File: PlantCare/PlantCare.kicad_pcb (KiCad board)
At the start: 2 copper layers, 27 parts, among them J1 USB4105-GF-A, SW1 PTS810_SJM_250_SMTR_LFS, SW2 PTS810_SJM_250_SMTR_LFS, U1 AMS1117-3.3, U2 ESP32-S3-WROOM-1-N16R2

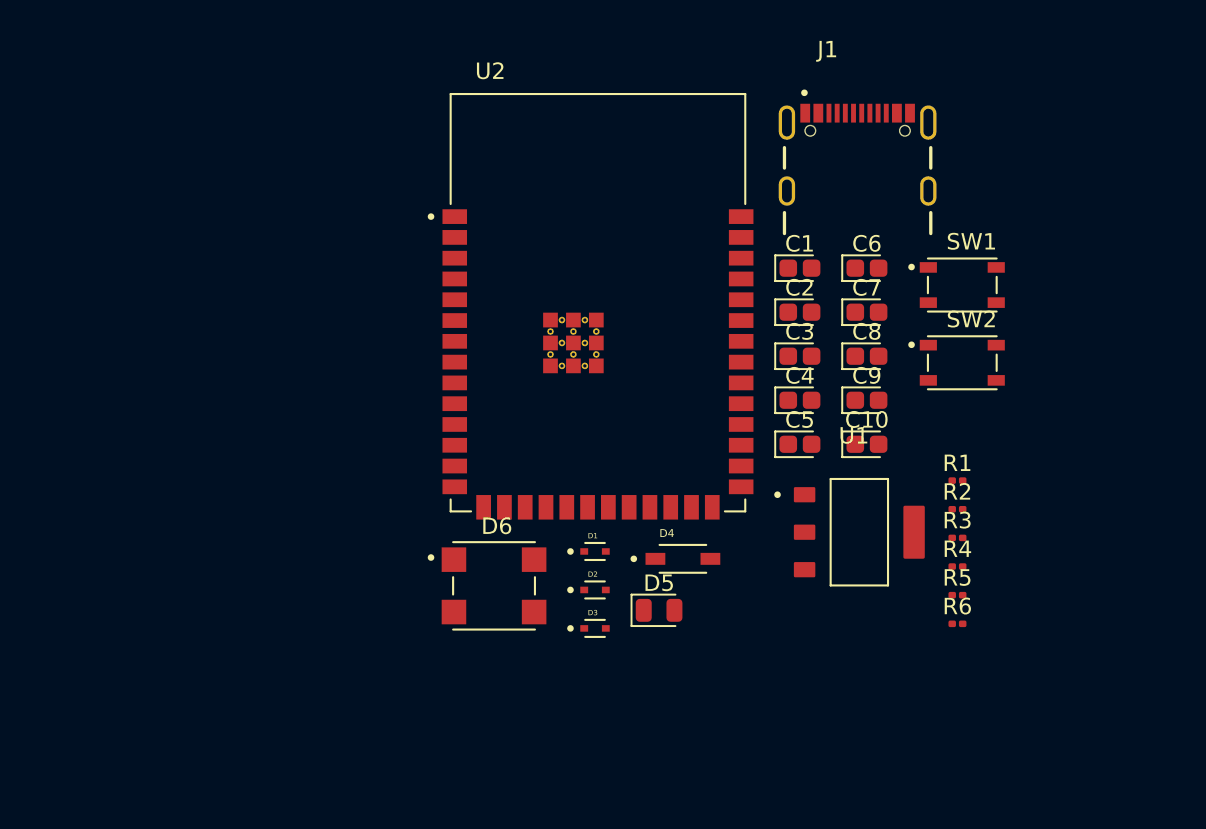
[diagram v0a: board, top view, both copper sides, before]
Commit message: Clear pcb
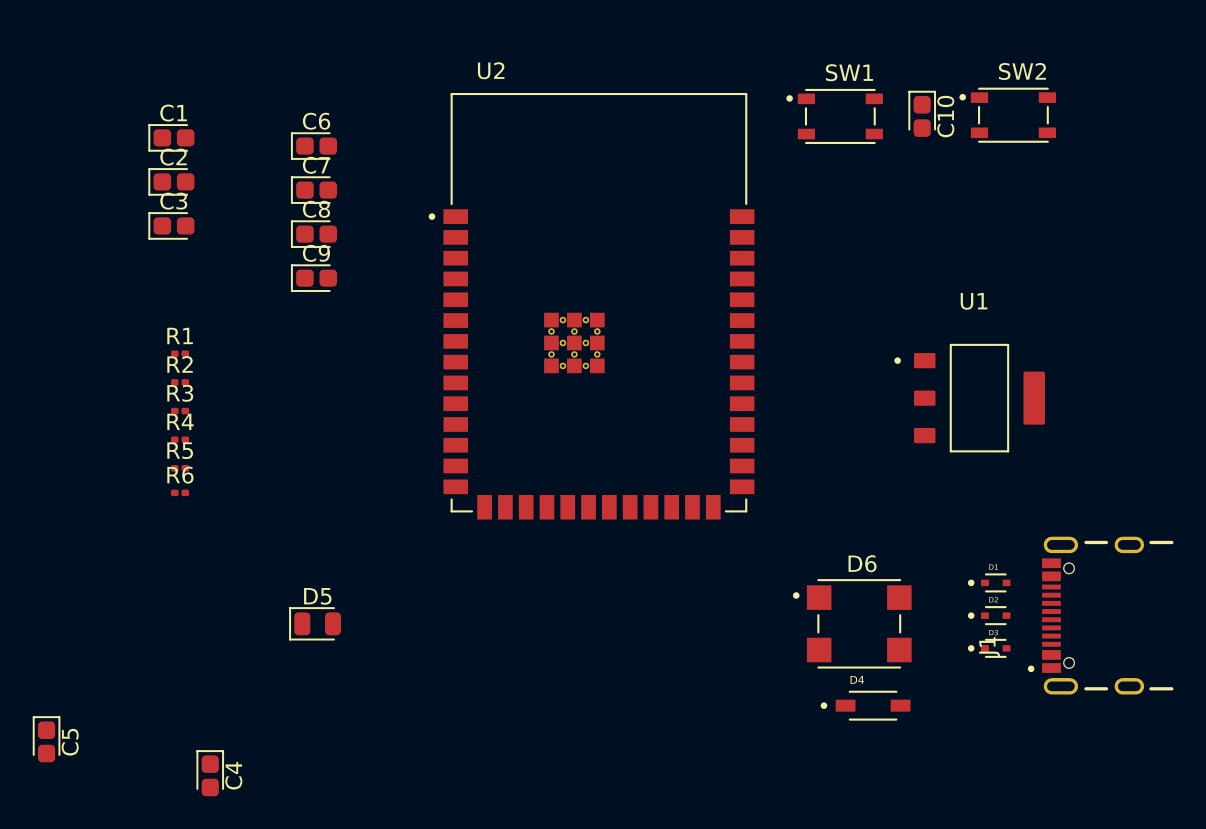
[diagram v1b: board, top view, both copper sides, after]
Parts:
- moved C5 49.5 mm to (111.5, 112.2), turned to -90 degrees
- moved R6 48.2 mm to (119.7, 97.0)
- moved R1 48.1 mm to (119.7, 88.5)
- moved R2 48.1 mm to (119.7, 90.2)
- moved R3 48.1 mm to (119.7, 92.0)
- moved R4 48.1 mm to (119.7, 93.8)
- moved R5 48.1 mm to (119.7, 95.5)
- moved C4 42.7 mm to (121.5, 114.3), turned to -90 degrees
- moved C3 39.1 mm to (119.3, 80.7)
- moved C1 39.1 mm to (119.3, 75.3)
- moved C2 39.1 mm to (119.3, 78.0)
- moved C8 34.4 mm to (128.0, 81.2)
- moved C9 34.4 mm to (128.0, 83.9)
- moved C6 34.4 mm to (128.0, 75.8)
- moved C7 34.4 mm to (128.0, 78.5)
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
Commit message: Fix pc
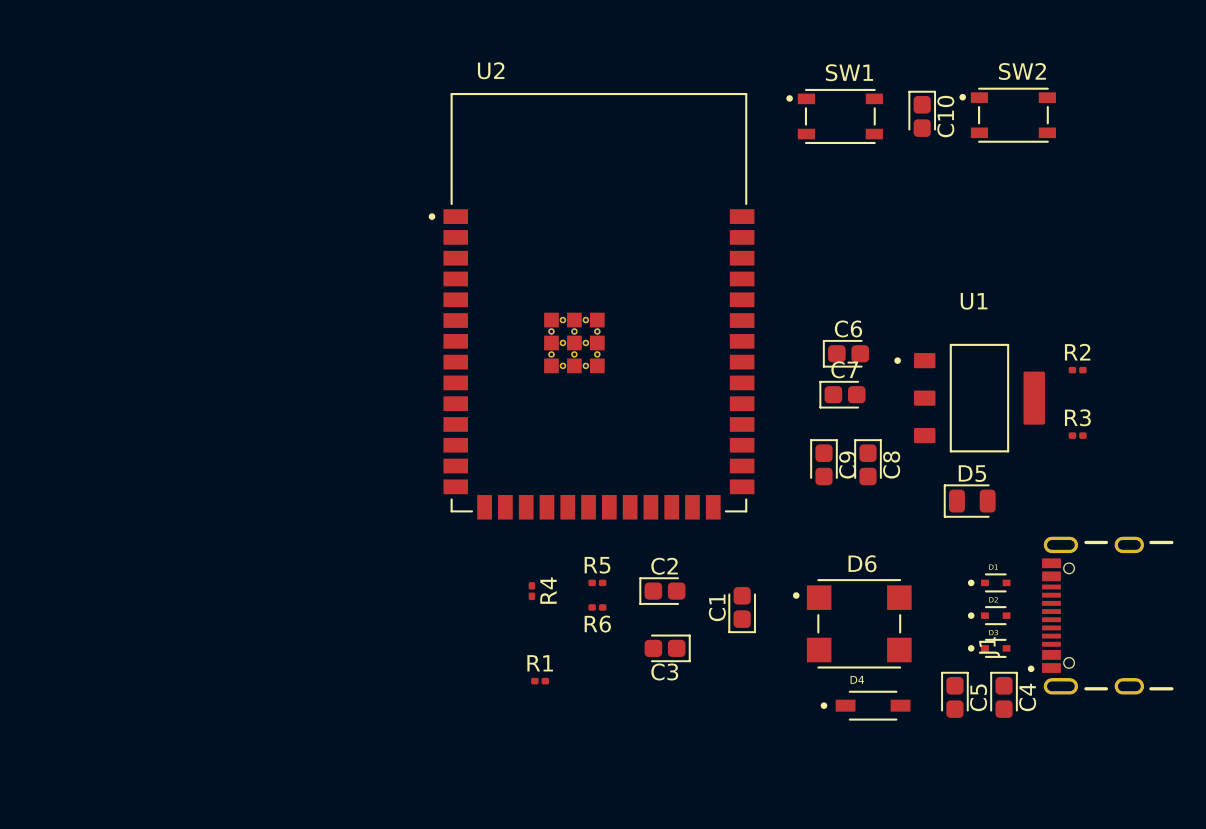
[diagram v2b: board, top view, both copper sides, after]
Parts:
- moved C5 55.6 mm to (167.0, 109.5)
- moved R3 54.9 mm to (174.5, 93.5)
- moved R2 54.9 mm to (174.5, 89.5)
- moved C4 48.7 mm to (170.0, 109.5)
- moved C1 45.0 mm to (154.0, 104.0), turned to 90 degrees
- moved D5 40.7 mm to (168.1, 97.5)
- moved C3 39.6 mm to (149.3, 106.5), turned to 180 degrees
- moved C2 39.1 mm to (149.3, 103.0)
- moved C8 36.5 mm to (161.7, 95.3), turned to -90 degrees
- moved C6 34.9 mm to (160.5, 88.5)
- moved C7 34.6 mm to (160.3, 91.0)
- moved C9 33.0 mm to (159.0, 95.3), turned to -90 degrees
- moved R1 29.7 mm to (141.7, 108.5)
- moved R5 26.4 mm to (145.2, 102.5)
- moved R6 26.4 mm to (145.2, 104.0), turned to 180 degrees
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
